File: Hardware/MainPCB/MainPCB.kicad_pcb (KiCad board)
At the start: 2 copper layers, 99.1 x 99.1 mm, 53 parts, among them J1 USB_B_Micro, J2 Conn_01x11, J3 UART, Q1 NTR2101P, Q2 FDS9926A, U1 BQ24075, U2 BQ29700, U3 TLV75533PDBV, U4 ESP32-WROOM-32D, U5 TPS22919, U6 TPS22919, U7 TPS22919

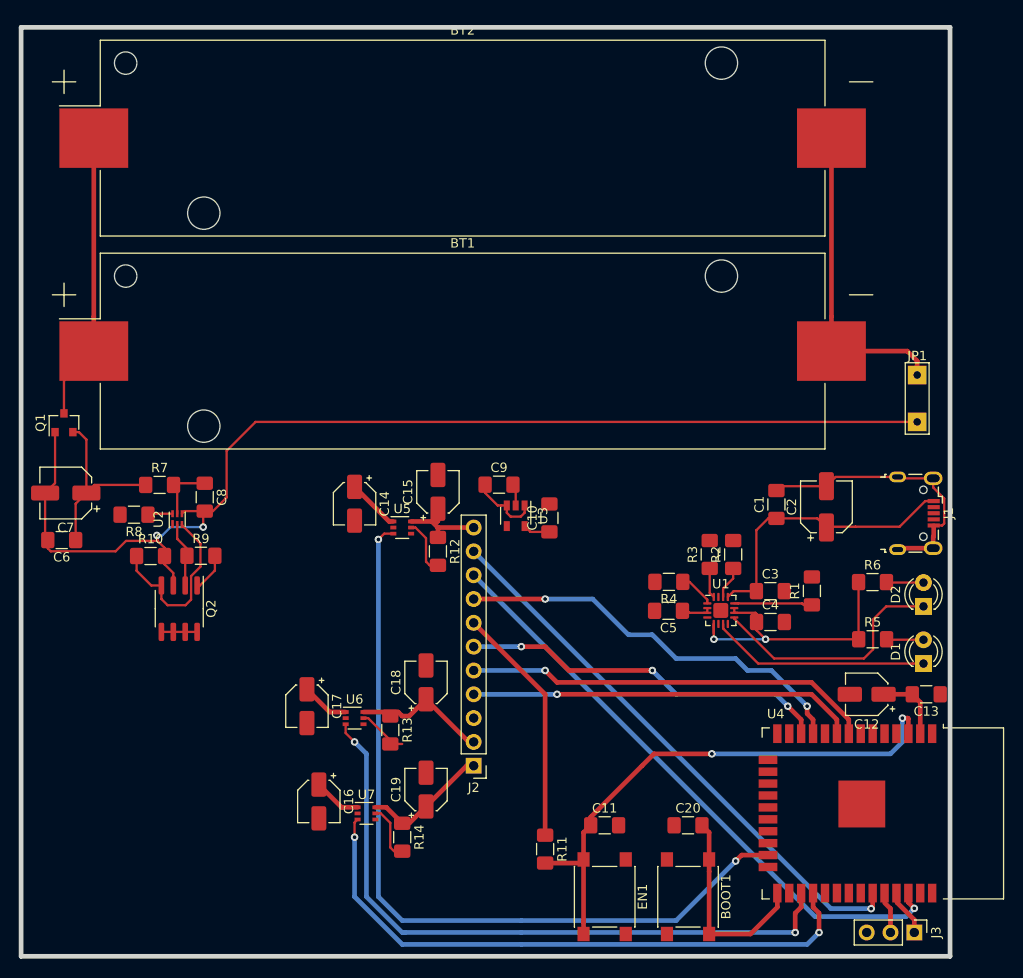
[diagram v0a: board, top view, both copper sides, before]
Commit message: Finished MainPCB + generated gerber files + aanpassingen BOM
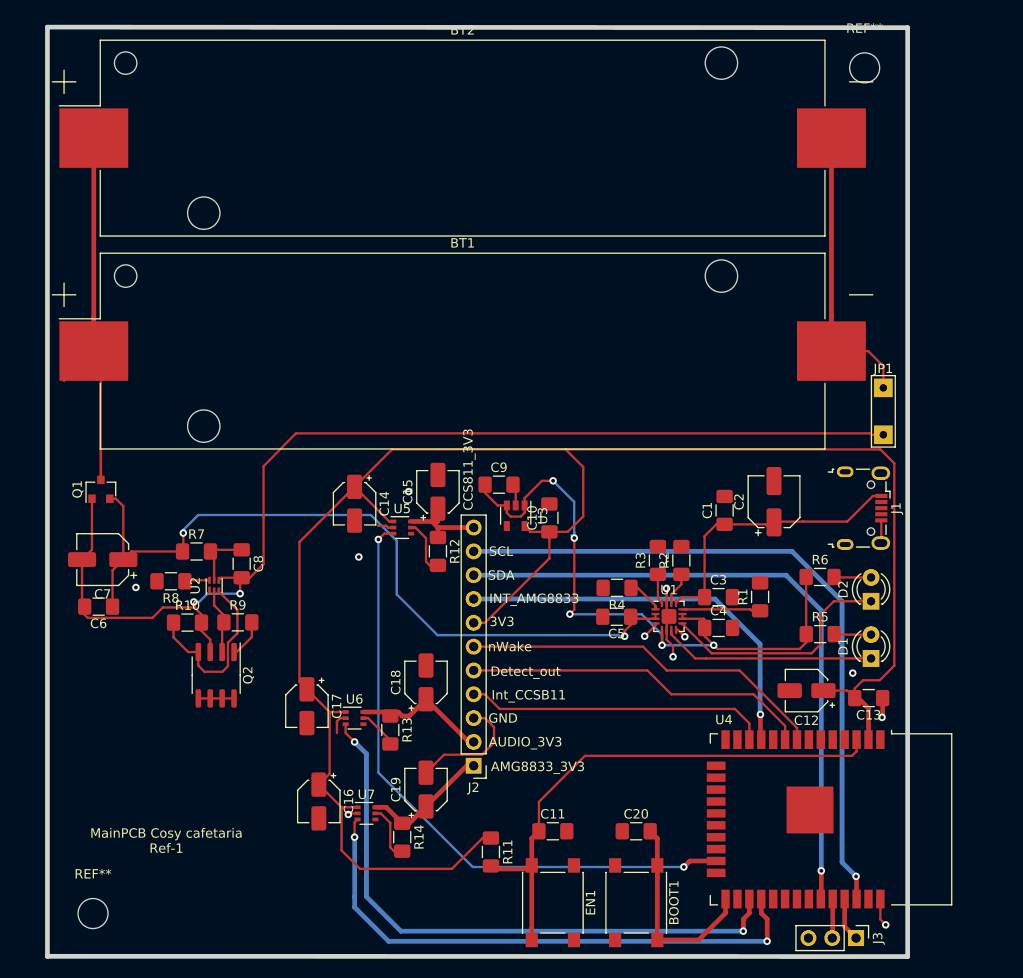
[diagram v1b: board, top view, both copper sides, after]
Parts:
- added REF**: MountingHole_3.2mm_M3, MountingHole:MountingHole_3.2mm_M3, F.Cu at (58.5, 130.1)
- added REF**: MountingHole_3.2mm_M3, MountingHole:MountingHole_3.2mm_M3, F.Cu at (140.8, 39.9)
- moved R9 8.12 mm to (73.9, 99.0)
- moved C8 8.12 mm to (74.3, 92.8)
- moved C6 8.12 mm to (59.1, 97.3)
- moved R8 8.12 mm to (66.8, 94.6)
- moved C7 8.12 mm to (59.5, 92.3)
- moved Q1 8.12 mm to (59.3, 84.8)
- moved Q2 8.12 mm to (71.6, 104.6)
- moved R10 8.12 mm to (68.5, 99.0)
- moved R7 8.12 mm to (69.5, 91.5)
- moved U2 8.12 mm to (71.4, 95.1)
- moved C12 6.43 mm to (134.6, 106.3)
- moved J3 6.24 mm to (139.8, 132.7)
- moved C13 6.15 mm to (141.2, 107.1)
- moved R11 5.79 mm to (100.9, 123.5)
- moved C2 5.61 mm to (131.1, 86.1)
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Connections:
- C3 pad 2: Net-(C3-Pad2) -> GND
- J2 pad 10: SDA -> SCL
- J2 pad 4: Detector_out -> Int_CCSB11
- J2 pad 5: nWake -> Detector_out
- J2 pad 6: Int_CCSB11 -> nWake
- J2 pad 9: SCL -> SDA
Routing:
- net +3V3: track 52.2 -> 195.9 mm
- net VDD1: track 23.0 -> 84.1 mm, vias 0 -> 2
- net VDD2: track 37.7 -> 71.2 mm, vias 2 -> 5
- net PowerS1: track 85.4 -> 67.2 mm
- net +BATT: track 30.7 -> 44.7 mm
- net SCL: track 64.3 -> 73.9 mm
- net SDA: track 59.9 -> 69.4 mm
- net Int_CCSB11: track 39.6 -> 32.4 mm, vias 3 -> 0
- net PowerS2: track 71.1 -> 64.7 mm
- net GND: track 36.6 -> 42.7 mm, vias 0 -> 11
- net PowerS3: track 65.0 -> 59.5 mm
- net nWake: track 43.7 -> 39.3 mm, vias 1 -> 0
- net Detector_out: track 41.4 -> 37.1 mm, vias 1 -> 0
- net Net-(BT1-Pad2): track 33.8 -> 31.2 mm
- net -BATT: track 123.8 -> 121.9 mm
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- added copper zone on B.Cu, net GND
- added copper zone on F.Cu, net GND
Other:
- board size 99.1 x 99.1 mm -> 91.7 x 99.1 mm
- board text added: "3V3"
- board text added: "AMG8833_3V3"
- board text added: "AUDIO_3V3"
- board text added: "CCS811_3V3"
- board text added: "Detect_out"
- board text added: "GND"
- board text added: "INT_AMG8833"
- board text added: "Int_CCSB11"
- board text added: "MainPCB Cosy cafetaria Ref-1"
- board text added: "SCL"
- board text added: "SDA"
- board text added: "nWake"
